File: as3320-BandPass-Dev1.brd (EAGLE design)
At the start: 70.8 x 128.6 mm, 92 parts, among them IC1 CEM3320, IC2 TL074D, IC3 LM4040 5.0V, IC4 TL074D, IC5 TL072D

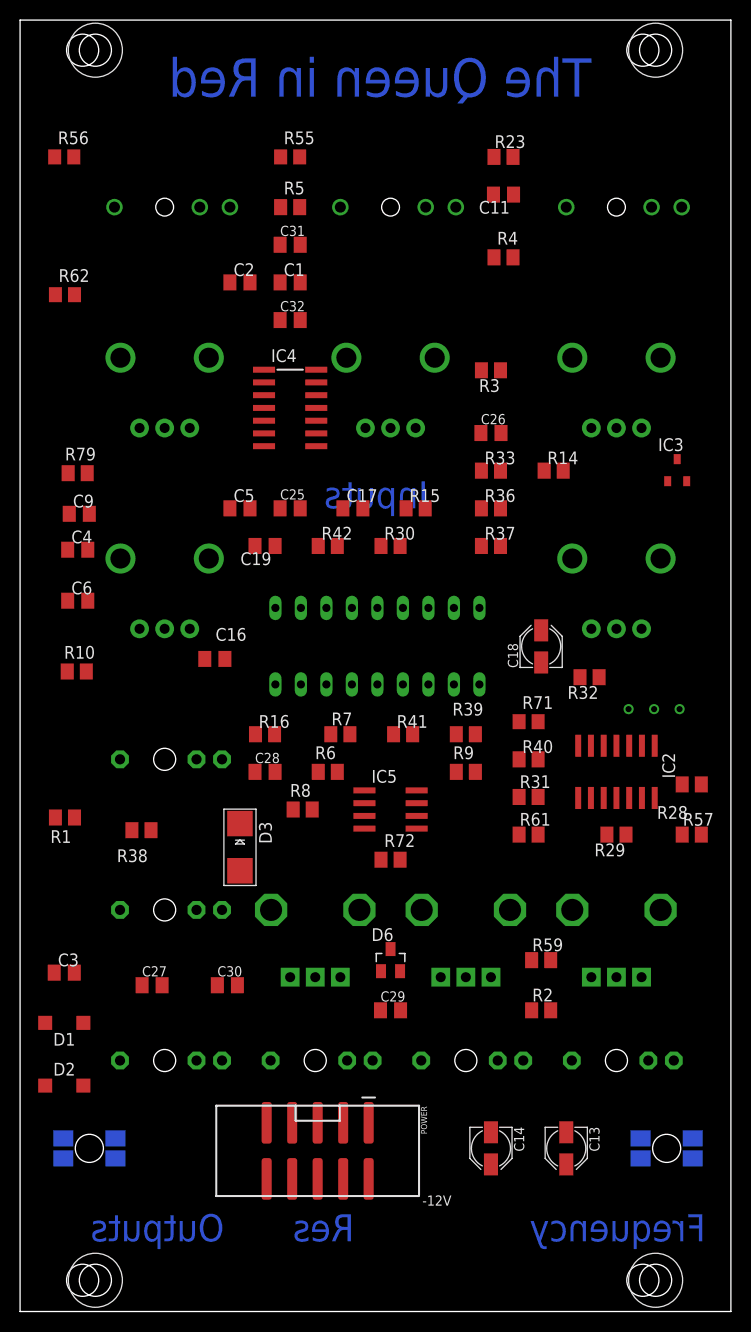
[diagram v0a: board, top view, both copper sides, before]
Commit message: Routed
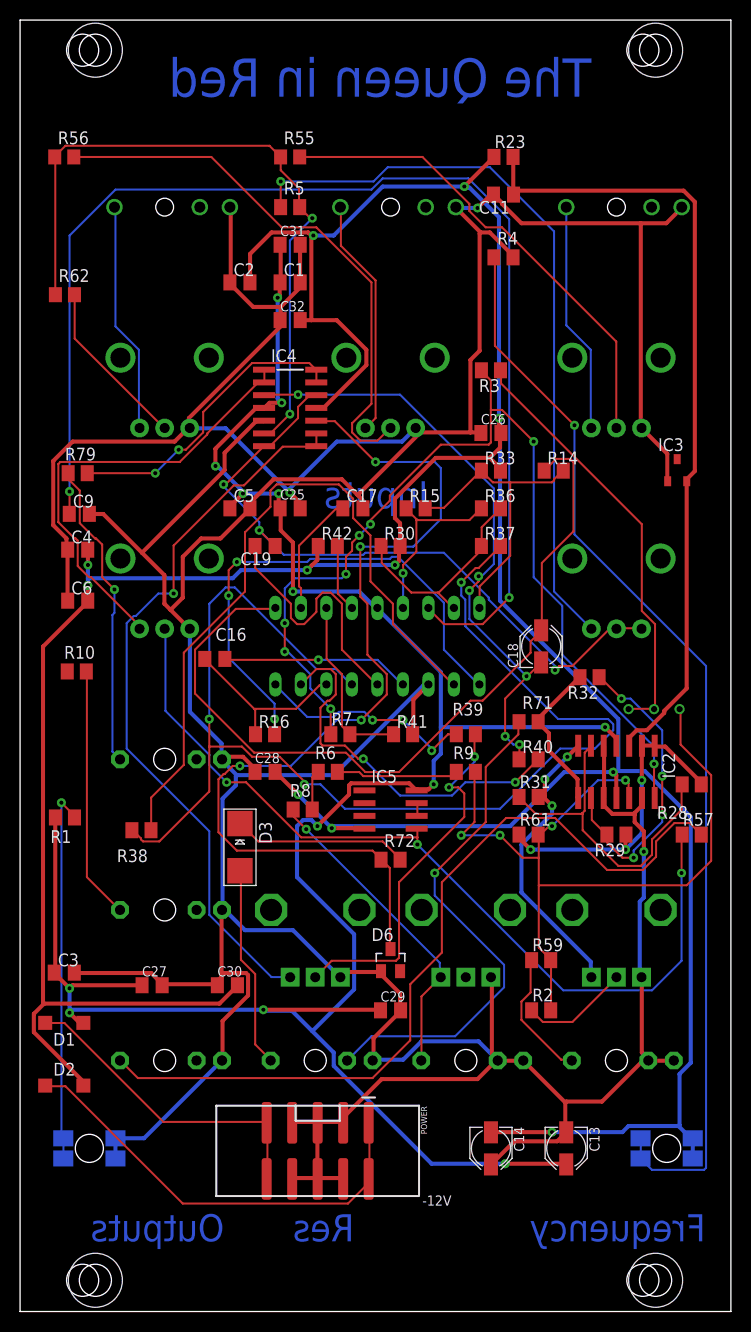
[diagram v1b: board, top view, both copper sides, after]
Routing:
- net GND: track 0.00 -> 526.6 mm, vias 0 -> 3
- net -12V: track 0.00 -> 365.3 mm, vias 0 -> 11
- net 12V: track 0.00 -> 233.8 mm, vias 0 -> 13
- net N$36: track 0.00 -> 123.4 mm, vias 0 -> 3
- net N$30: track 0.00 -> 123.1 mm, vias 0 -> 2
- net N$74: track 0.00 -> 108.5 mm, vias 0 -> 1
- net N$3: track 0.00 -> 98.8 mm, vias 0 -> 8
- net N$89: track 0.00 -> 96.7 mm, vias 0 -> 4
- net N$11: track 0.00 -> 86.9 mm, vias 0 -> 3
- net O2: track 0.00 -> 82.2 mm
- net N$12: track 0.00 -> 81.2 mm, vias 0 -> 4
- net -5VIN: track 0.00 -> 80.1 mm
- net N$31: track 0.00 -> 80.0 mm
- net N$20: track 0.00 -> 74.1 mm, vias 0 -> 1
- net RESONANCE_IN2: track 0.00 -> 73.3 mm, vias 0 -> 1
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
